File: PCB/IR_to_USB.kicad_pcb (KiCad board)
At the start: 2 copper layers, 120.7 x 44.4 mm, 5 parts, among them U1 STM32F070CBT6

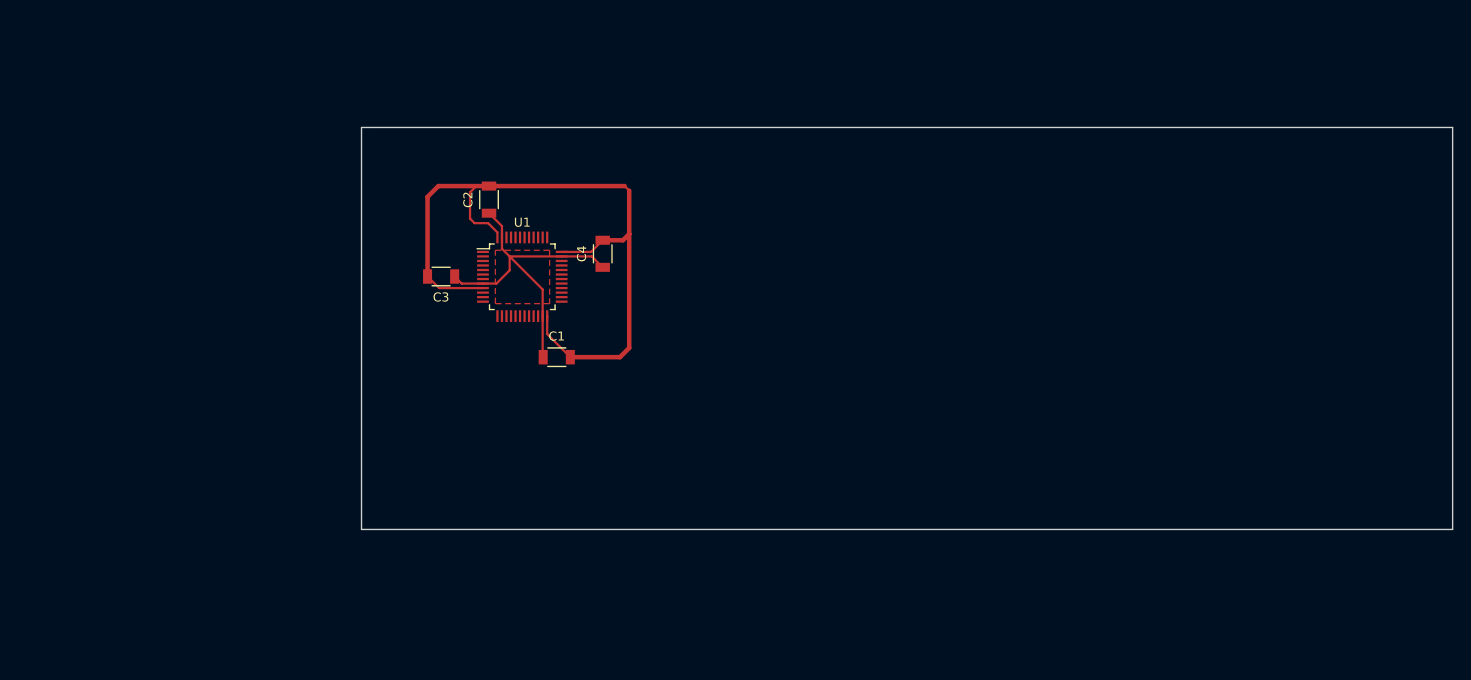
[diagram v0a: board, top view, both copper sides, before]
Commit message: PCB in progress
Signed-off-by: denis-m-tyurin <denis.m.turin@gmail.com>
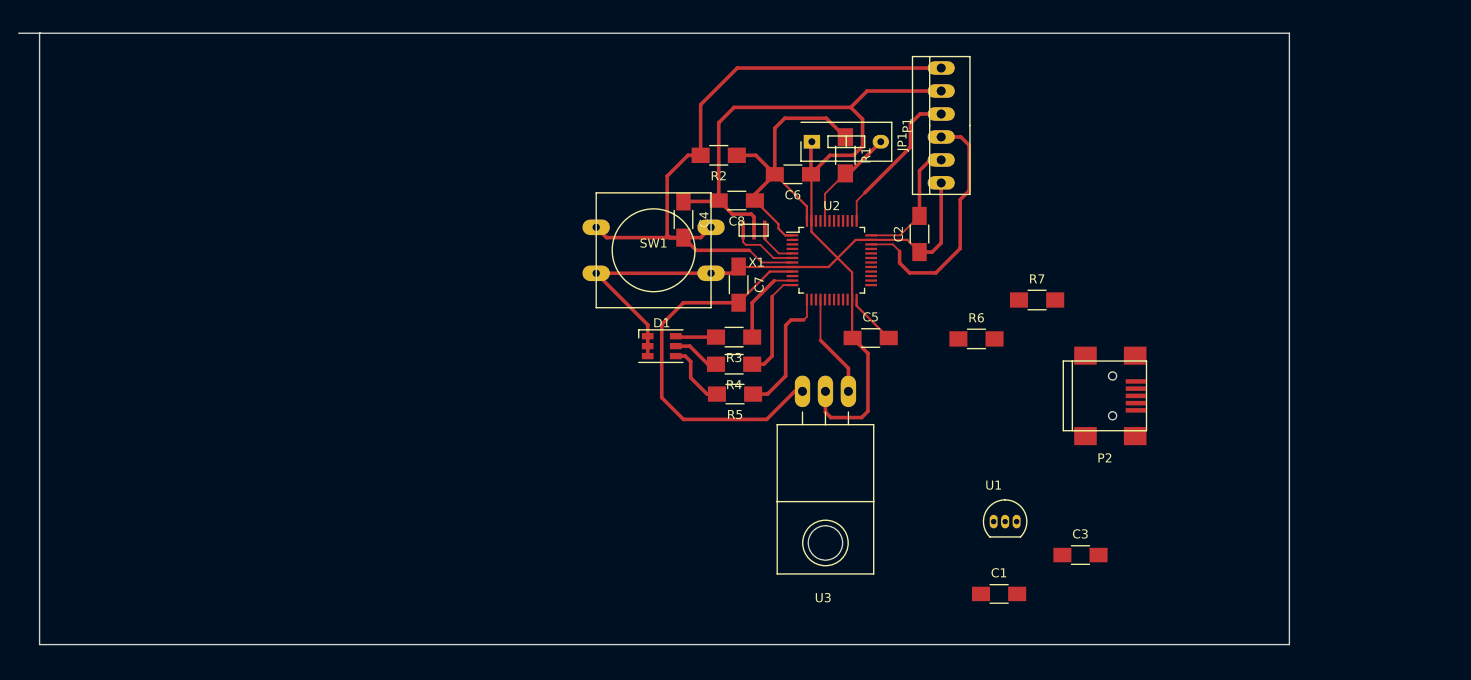
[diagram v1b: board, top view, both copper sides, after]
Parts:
- added C5: 100 nF, Capacitors_SMD:C_1206_HandSoldering, F.Cu at (145.2, 94.4)
- added C6: 100 nF, Capacitors_SMD:C_1206_HandSoldering, F.Cu at (136.6, 76.3)
- added C7: 100 nF, Capacitors_SMD:C_1206_HandSoldering, F.Cu at (130.6, 88.5)
- added C8: 100 nF, Capacitors_SMD:C_1206_HandSoldering, F.Cu at (130.4, 79.2)
- added D1: LED_RGB, LEDs:LED_RGB_PLLC-6, F.Cu at (122.1, 95.3)
- added JP1: JUMPER, Buttons_Switches_ThroughHole:SW_DIP_x1_Slide, F.Cu at (138.7, 72.7)
- added P1: CONN_01X06, Connect:PINHEAD1-6, F.Cu at (153.0, 70.9)
- added P2: USB_OTG, Connect:USB_Mini-B, F.Cu at (171.1, 100.8)
- added R1: 10K, Resistors_SMD:R_1206_HandSoldering, F.Cu at (142.4, 74.2)
- added R2: 10K, Resistors_SMD:R_1206_HandSoldering, F.Cu at (128.4, 74.2)
- added R3: 62, Resistors_SMD:R_1206_HandSoldering, F.Cu at (130.1, 94.3)
- added R4: 5, Resistors_SMD:R_1206_HandSoldering, F.Cu at (130.1, 97.3)
- added R5: 5, Resistors_SMD:R_1206_HandSoldering, F.Cu at (130.2, 100.6)
- added R6: 33, Resistors_SMD:R_1206_HandSoldering, F.Cu at (156.9, 94.5)
- added R7: 33, Resistors_SMD:R_1206_HandSoldering, F.Cu at (163.6, 90.2)
- added SW1: SW_PUSH, Buttons_Switches_ThroughHole:SW_PUSH-12mm, F.Cu at (121.2, 84.7)
- added U2: STM32F070CBT6, Housings_QFP:LQFP-48_7x7mm_Pitch0.5mm, F.Cu at (140.9, 85.8)
- added U3: TSOP48, TO_SOT_Packages_THT:TO-220_Neutral123_Horizontal_LargePads, F.Cu at (140.2, 100.3)
- added X1: CRYSTAL_SMD, Footprint_lib:CSTCE_G_Murata_Resonator, F.Cu at (131.1, 81.7)
- C1, C2, C4: footprint Capacitors_SMD:C_1206 -> Capacitors_SMD:C_1206_HandSoldering
- C3: value 100 nF -> 330 nF; footprint Capacitors_SMD:C_1206 -> Capacitors_SMD:C_1206_HandSoldering
- U1: value STM32F070CBT6 -> L78L; footprint Housings_QFP:LQFP-48_7x7mm_Pitch0.5mm -> TO_SOT_Packages_THT:TO-92_Inline_Narrow_Oval
- moved C3 77.1 mm to (168.4, 118.4), turned to 0 degrees
- moved U1 58.7 mm to (158.8, 114.7)
- moved C1 55.5 mm to (159.4, 122.7)
- moved C2 47.8 mm to (150.6, 82.9)
- moved C4 9.70 mm to (124.5, 81.3), turned to 270 degrees
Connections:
- C1 pad 1: Earth -> +3V3
- C1 pad 2: +3V3 -> Earth
- C3 pad 1: Earth -> +5V
- C3 pad 2: +3V3 -> Earth
- C4 pad 2: +3V3 -> Net-(C4-Pad2)
- U1 pad 1: Net-(U1-Pad1) -> +3V3
- U1 pad 2: Net-(U1-Pad2) -> Earth
- U1 pad 3: Net-(U1-Pad3) -> +5V
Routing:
- net Earth: track 38.3 -> 155.6 mm
- net Net-(C4-Pad2): track 0.00 -> 73.8 mm
- net Net-(P1-Pad3): track 0.00 -> 28.3 mm
- net Net-(P1-Pad4): track 0.00 -> 17.1 mm
- net Net-(R5-Pad1): track 0.00 -> 14.7 mm
- net +3V3: track 85.8 -> 98.4 mm
- net Net-(R4-Pad1): track 0.00 -> 11.9 mm
- net Net-(JP1-Pad2): track 0.00 -> 11.6 mm
- net Net-(U2-Pad16): track 0.00 -> 11.4 mm
- net Net-(R3-Pad1): track 0.00 -> 9.26 mm
- net Net-(U2-Pad6): track 0.00 -> 7.51 mm
- net Net-(D1-Pad4): track 0.00 -> 7.34 mm
- net Net-(D1-Pad5): track 0.00 -> 5.28 mm
- net Net-(U2-Pad5): track 0.00 -> 4.73 mm
- net Net-(D1-Pad6): track 0.00 -> 4.49 mm
- removed copper zone on F.Cu, net Earth
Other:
- board size 120.7 x 44.4 mm -> 140.5 x 67.6 mm

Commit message: First PCB draft
Signed-off-by: denis-m-tyurin <denis.m.turin@gmail.com>
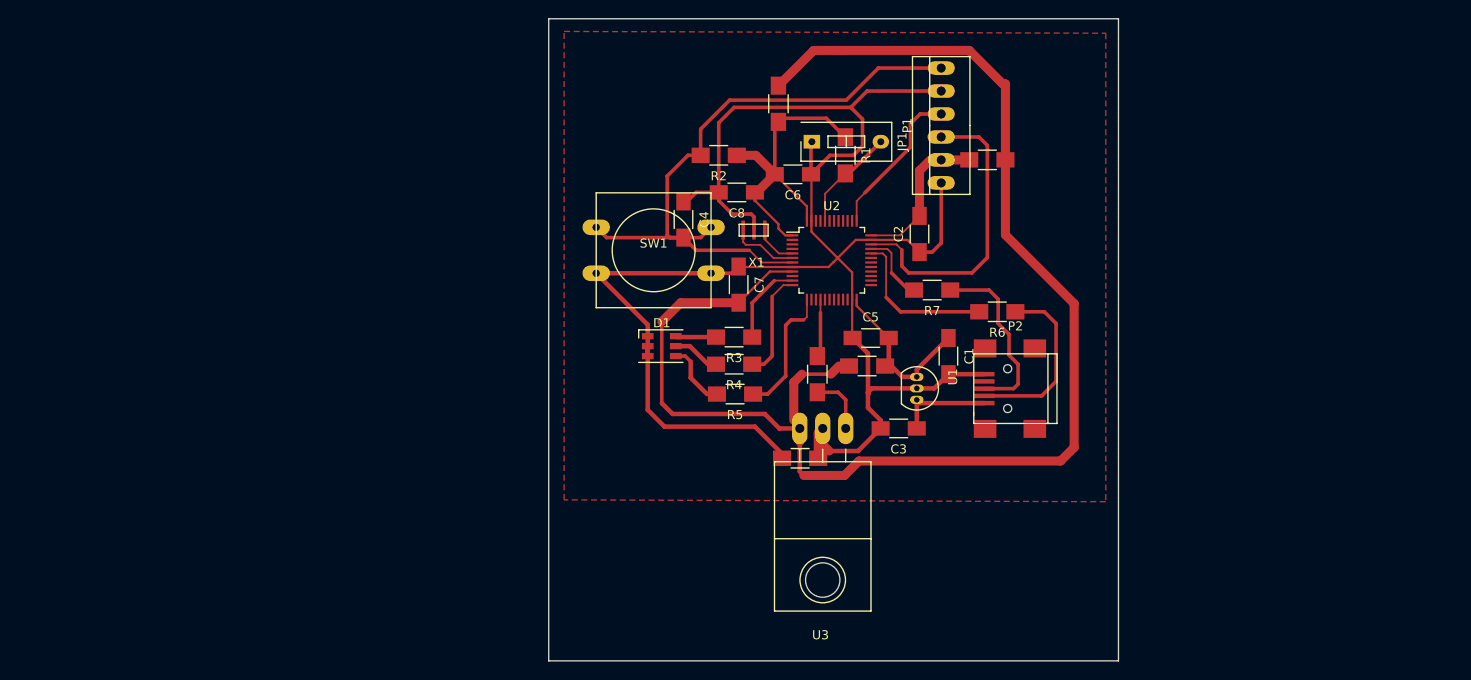
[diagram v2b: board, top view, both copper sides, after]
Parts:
- added  : R0, Resistors_SMD:R_1206_HandSoldering, F.Cu at (137.4, 107.7)
- added  : R0, Resistors_SMD:R_1206_HandSoldering, F.Cu at (135.0, 68.5)
- added  : R0, Resistors_SMD:R_1206_HandSoldering, F.Cu at (158.1, 74.7)
- added  : R0, Resistors_SMD:R_1206_HandSoldering, F.Cu at (139.3, 98.4)
- added  : R0, Resistors_SMD:R_1206_HandSoldering, F.Cu at (144.8, 97.5)
- moved C1 26.9 mm to (153.8, 96.4), turned to 270 degrees
- moved C3 24.5 mm to (148.3, 104.4), turned to 180 degrees
- moved U1 18.1 mm to (150.3, 98.7), turned to 270 degrees
- moved R7 11.7 mm to (152.0, 89.1), turned to 180 degrees
- moved P2 9.93 mm to (161.2, 100.0), turned to 180 degrees
- moved U3 4.11 mm to (139.9, 104.4)
- moved R6 3.78 mm to (159.2, 91.5), turned to 180 degrees
- moved C8 0.90 mm to (130.4, 78.3)
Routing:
- net +3V3: track 98.4 -> 234.7 mm
- net Earth: track 155.6 -> 201.9 mm
- net Net-(P2-Pad2): track 0.00 -> 20.1 mm
- net Net-(P2-Pad3): track 0.00 -> 20.0 mm
- net Net-(R6-Pad2): track 0.00 -> 17.3 mm
- net +5V: track 0.00 -> 10.8 mm
- net Net-(R7-Pad2): track 0.00 -> 7.92 mm
- net Net-(P1-Pad3): track 28.3 -> 33.9 mm
- net Net-(U2-Pad16): track 11.4 -> 13.2 mm
- net Net-(C4-Pad2): track 73.8 -> 72.6 mm
- added copper zone on F.Cu, net Earth
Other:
- board size 140.5 x 67.6 mm -> 63 x 71 mm
- rule trace_min: 0.01 -> 0.2
